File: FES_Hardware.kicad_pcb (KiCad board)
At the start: 2 copper layers, 57 parts, among them J1 Screw_Terminal_01x02, Q1 STD5N20L, Q2 STD5N20L, Q3 STD5N20L, Q4 STD5N20L, SW1 SW_Rotary_1x8_MP, U1 LM2586S, U2 TPS63802DLAR, U3 ESP32-DEVKITC-32UE, U4 IRS2005M, U5 IRS2005M

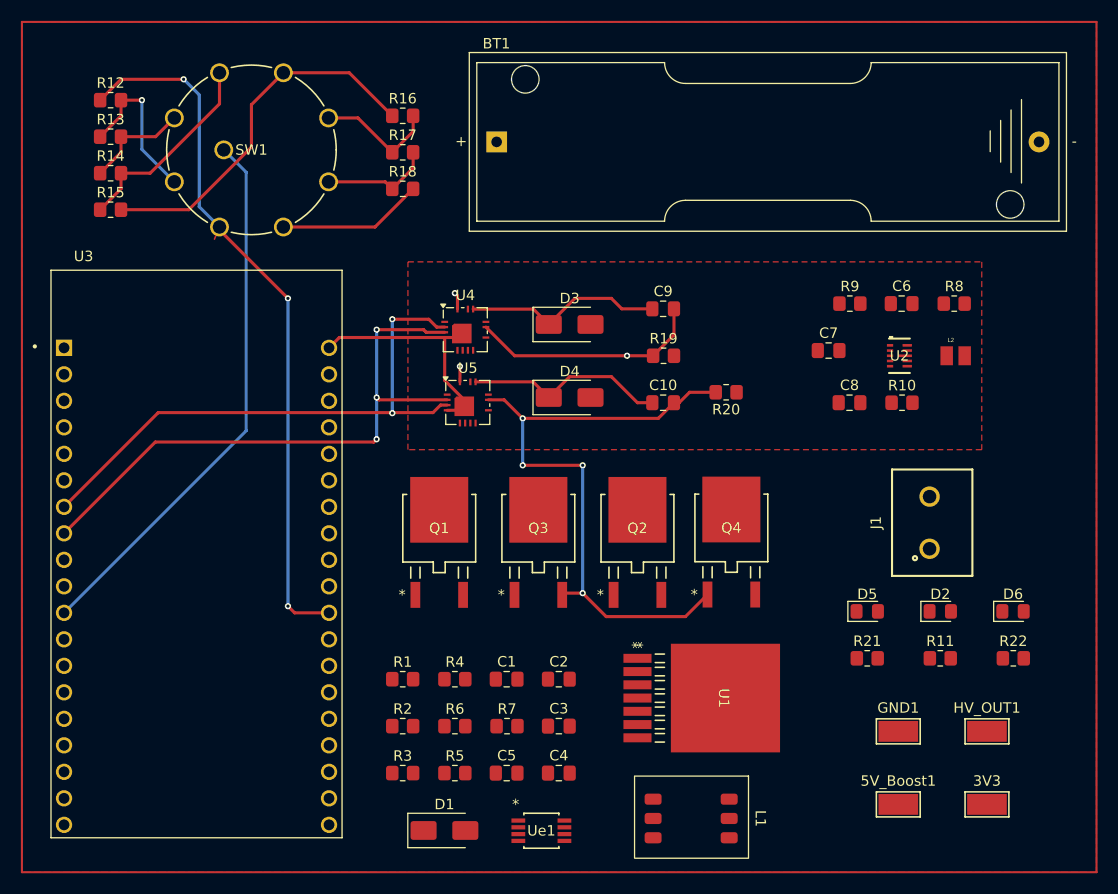
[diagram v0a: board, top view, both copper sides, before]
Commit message: ryanPCB branch commit for pcb layout
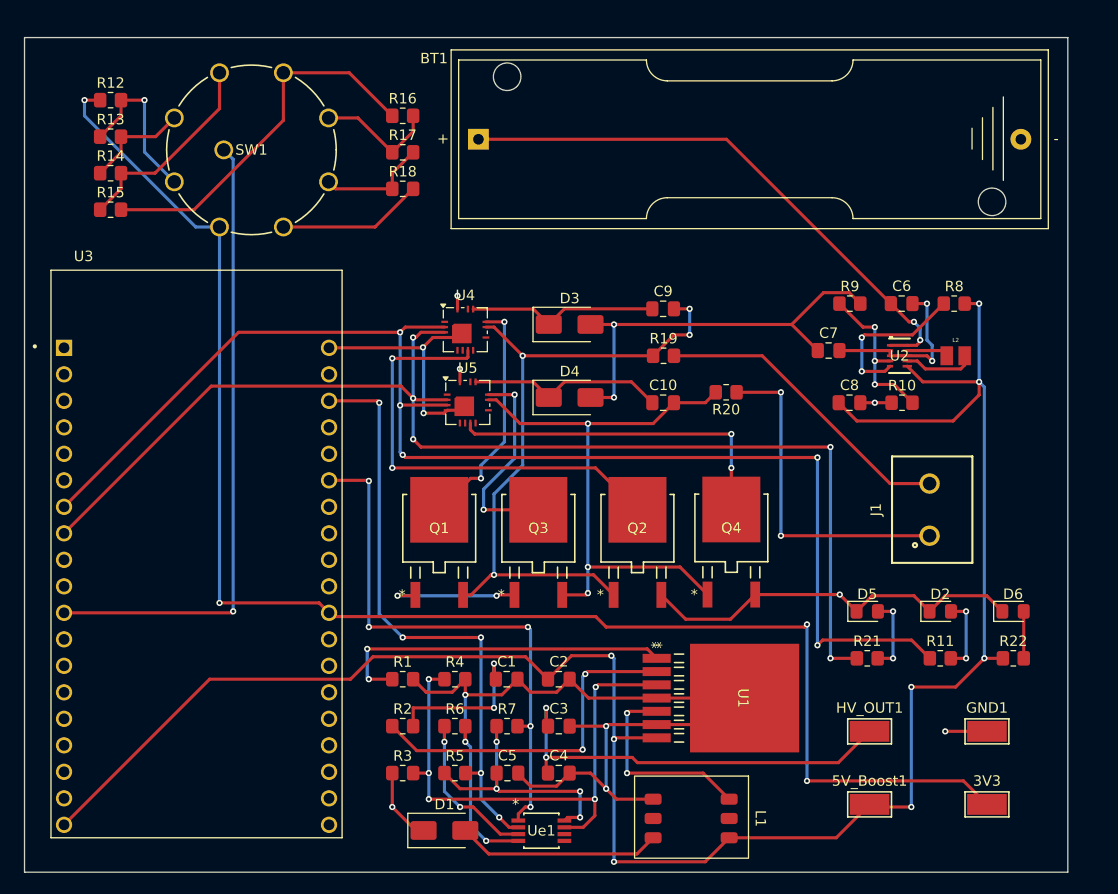
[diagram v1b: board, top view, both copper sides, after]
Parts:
- moved HV_OUT1 11.2 mm to (166.8, 142.0)
- moved GND1 8.50 mm to (178.0, 142.0)
- moved 5V_Boost1 2.75 mm to (166.8, 149.0)
- moved U1 1.84 mm to (154.6, 138.8)
- moved BT1 1.76 mm to (129.3, 85.2)
- moved J1 1.25 mm to (172.5, 120.8)
- moved C5 0.07 mm to (132.0, 146.0)
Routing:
- net +5V: track 3.13 -> 239.7 mm, vias 2 -> 12
- net GND: track 36.4 -> 197.8 mm, vias 0 -> 12
- net ROT_3V3: track 67.4 -> 146.9 mm, vias 3 -> 4
- net DRV_A: track 55.1 -> 129.6 mm, vias 2 -> 5
- net DRV_B: track 57.7 -> 119.3 mm, vias 3 -> 5
- net ESP32_SCL: track 0.00 -> 57.5 mm, vias 0 -> 5
- net Net-(BT1-+): track 0.00 -> 54.4 mm, vias 0 -> 2
- net ESP32_SDA: track 0.00 -> 53.8 mm, vias 0 -> 5
- net Net-(U1-FB): track 0.00 -> 52.1 mm, vias 0 -> 5
- net HV_OUT: track 0.00 -> 47.8 mm, vias 0 -> 3
- net Net-(Q2-G): track 0.00 -> 43.6 mm, vias 0 -> 2
- net Net-(Q1-S): track 22.5 -> 63.6 mm, vias 1 -> 4
- net Net-(U1-COMP): track 0.00 -> 33.6 mm, vias 0 -> 2
- net Net-(U1-~ON/OFF): track 0.00 -> 33.3 mm, vias 0 -> 2
- net Net-(Q4-G): track 0.00 -> 33.1 mm, vias 0 -> 2
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- added copper zone on In2.Cu, net +5V
- added copper zone on In1.Cu, net GND
- added copper zone on In2.Cu, net HV_OUT
- removed copper zone on F.Cu, net +5V
- removed copper zone on B.Cu, net GND
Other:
- board outline added: 100 x 80 mm
- copper layers 2 -> 4
